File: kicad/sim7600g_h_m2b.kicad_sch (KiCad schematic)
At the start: 35 parts, among them IC2 TXB0102DCUR, IC5 TXB0102DCUR, J2 APCI0105-P001A, J3 SMN-303, U2 MMBT3904TT1G

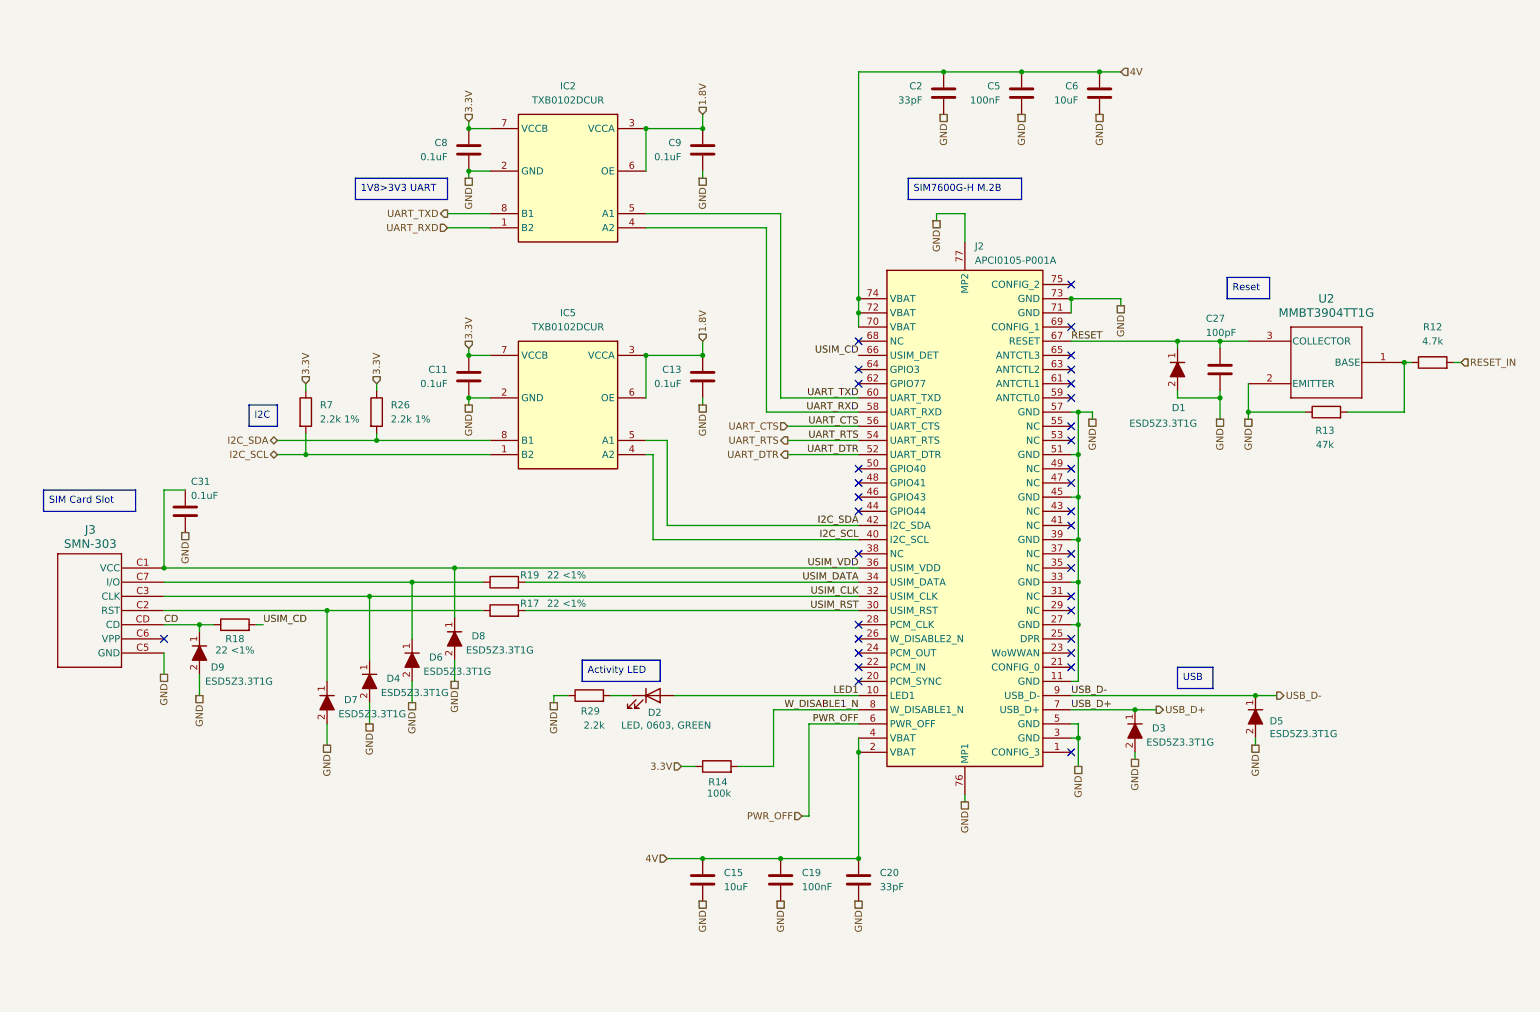
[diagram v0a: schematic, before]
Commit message: finish first pcb revision
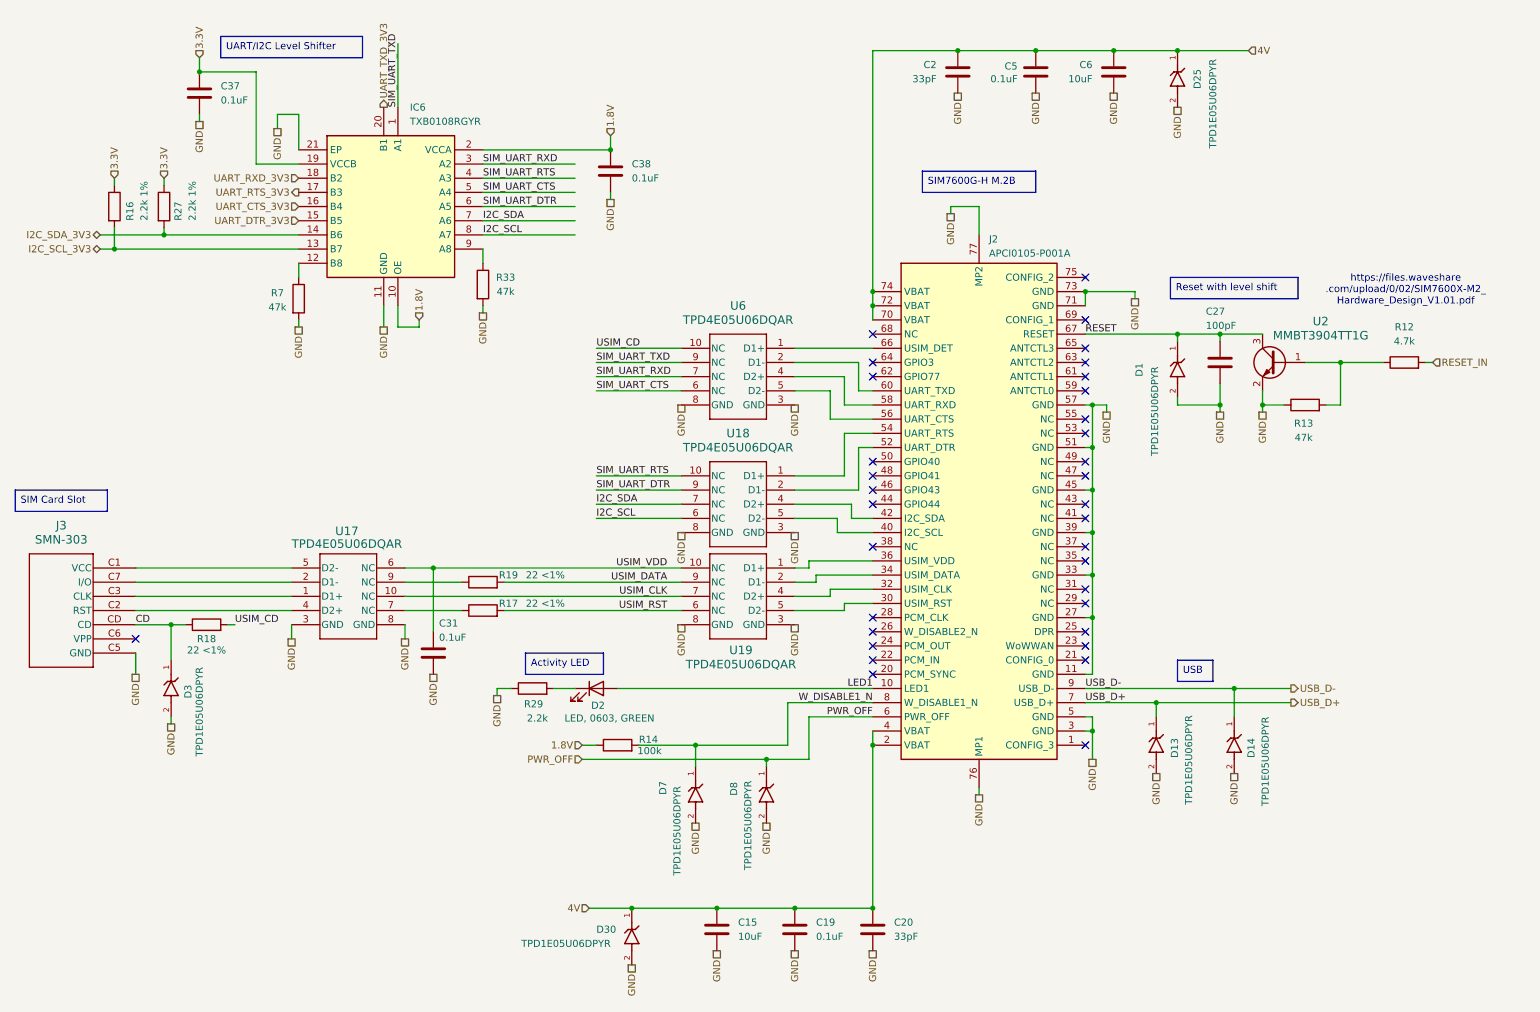
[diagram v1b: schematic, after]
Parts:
- removed C11, C13, C8, C9: 0.1uF, symbol Device:C
- removed D1, D3, D4, D5, D6, D7, D8, D9: ESD5Z3.3T1G, symbol ESD5Z3_3T1G:ESD5Z3.3T1G
- removed IC2, IC5: TXB0102DCUR, symbol TXB0102DCUR:TXB0102DCUR
- removed R26: 2.2k 1%, symbol Device:R
- added C37, C38: 0.1uF, Capacitor_SMD:C_0201_0603Metric, symbol Device:C
- added D1, D13, D14, D25, D3, D30, D7, D8: TPD1E05U06DPYR, TPD1E05U06DPYR:SON65P60X100X45-2N, symbol TPD1E05U06DPYR:TPD1E05U06DPYR
- added IC6: TXB0108RGYR, TXB0108RGYR:SN74LVC541ARGYR, symbol TXB0108RGYR:TXB0108RGYR
- added R16, R27: 2.2k 1%, Resistor_SMD:R_0201_0603Metric, symbol Device:R
- added R33: 47k, Resistor_SMD:R_0201_0603Metric, symbol Device:R
- added U17, U18, U19, U6: TPD4E05U06DQAR, TPD4E05U06DQAR:DQA0010A, symbol TPD4E05U06DQAR:TPD4E05U06DQAR
- C15, C6: footprint (none) -> Capacitor_SMD:C_0603_1608Metric
- C19, C5: value 100nF -> 0.1uF; footprint (none) -> Capacitor_SMD:C_0402_1005Metric
- C2, C20: footprint (none) -> Capacitor_SMD:C_0402_1005Metric
- C27, C31: footprint (none) -> Capacitor_SMD:C_0201_0603Metric
- J2: footprint (none) -> APCI0105-P001A:APCI0105P001A
- J3: footprint (none) -> SMN-303:SMN-303_XNP
- R12, R13, R17, R18, R19: footprint (none) -> Resistor_SMD:R_0201_0603Metric
- R7: value 2.2k 1% -> 47k; footprint (none) -> Resistor_SMD:R_0201_0603Metric
- U2: footprint (none) -> MMBT3904TT1G:SOT-416_1P65X0P9_ONS-L
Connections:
- net 1.8V: now also R14.1, C38.1, IC6.10 (OE), IC6.2 (VCCA)
- net 3.3V: now also C37.1, IC6.19 (VCCB), R16.1, R27.1; no longer R14.1, R7.1
- net 4V: now also D25.1, D30.1
- net CD: now also D3.1
- net GND: now also R7.2, C37.2, C38.2, D1.2, D13.2, D14.2, D25.2, D3.2, D30.2, D7.2, D8.2, IC6.11 (GND), IC6.21 (EP), R33.2, U17.3 (GND), U17.8 (GND), U18.3 (GND), U18.8 (GND), U19.3 (GND), U19.8 (GND), U6.3 (GND), U6.8 (GND)
- net I2C_SCL: now also IC6.8 (A7), U18.6 (NC); no longer J2.40 (I2C_SCL), R7.2
- net I2C_SDA: now also IC6.7 (A6), U18.7 (NC); no longer J2.42 (I2C_SDA)
- net PWR_OFF: now also D8.1
- net RESET: now also D1.1
- net USB_D+: now also D13.1
- net USB_D-: now also D14.1
- net USIM_CD: now also U6.10 (NC); no longer J2.66 (USIM_DET)
- net USIM_CLK: now also U17.10 (NC), U19.7 (NC); no longer J2.32 (USIM_CLK), J3.C3 (CLK)
- net USIM_DATA: now also U19.9 (NC); no longer J2.34 (USIM_DATA)
- net USIM_RST: now also U19.6 (NC); no longer J2.30 (USIM_RST)
- net USIM_VDD: now also U17.6 (NC), U19.10 (NC); no longer J2.36 (USIM_VDD), J3.C1 (VCC)
- net W_DISABLE1_N: now also D7.1
- net at J3.C2 (RST): now also U17.4 (D2+); no longer R17.1
- net at J3.C7 (I/O): now also U17.2 (D1-); no longer R19.1
- net UART_CTS: no longer names the net of J2.56 (UART_CTS)
- net UART_CTS: now also U6.5 (D2-)
- net UART_DTR: no longer names the net of J2.52 (UART_DTR)
- net UART_DTR: now also U18.2 (D1-)
- net UART_RTS: no longer names the net of J2.54 (UART_RTS)
- net UART_RTS: now also U18.1 (D1+)
- net UART_RXD: no longer names the net of J2.58 (UART_RXD)
- net UART_RXD: now also U6.4 (D2+)
- net UART_TXD: no longer names the net of J2.60 (UART_TXD)
- net UART_TXD: now also U6.2 (D1-)
- new net: J3.C1 (VCC), U17.5 (D2-)
- new net: J3.C3 (CLK), U17.1 (D1+)
- new net: J2.42 (I2C_SDA), U18.4 (D2+)
- new net: J2.40 (I2C_SCL), U18.5 (D2-)
- new net: R17.1, U17.7 (NC)
- new net: R19.1, U17.9 (NC)
- new net: J2.36 (USIM_VDD), U19.1 (D1+)
- new net: J2.34 (USIM_DATA), U19.2 (D1-)
- new net: J2.32 (USIM_CLK), U19.4 (D2+)
- new net: J2.30 (USIM_RST), U19.5 (D2-)
- new net: IC6.12 (B8), R7.1
- new net: IC6.9 (A8), R33.1
- new net: J2.66 (USIM_DET), U6.1 (D1+)
- new net I2C_SCL_3V3: IC6.13 (B7), R16.2
- new net I2C_SDA_3V3: IC6.14 (B6), R27.2
- new net SIM_UART_CTS: IC6.5 (A4), U6.6 (NC)
- new net SIM_UART_DTR: IC6.6 (A5), U18.9 (NC)
- new net SIM_UART_RTS: IC6.4 (A3), U18.10 (NC)
- new net SIM_UART_RXD: IC6.3 (A2), U6.7 (NC)
- new net SIM_UART_TXD: IC6.1 (A1), U6.9 (NC)
- new net UART_CTS_3V3: IC6.16 (B4)
- new net UART_DTR_3V3: IC6.15 (B5)
- new net UART_RTS_3V3: IC6.17 (B3)
- new net UART_RXD_3V3: IC6.18 (B2)
- new net UART_TXD_3V3: IC6.20 (B1)
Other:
- note added: "https://files.waveshare .com/upload/0/02/SIM7600X-M2_ Hardware_Design_V1.01.pdf"
- moved on the sheet: C15, C19, C2, C20, C27, C31, C5, C6, D2, J2, J3, R12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
